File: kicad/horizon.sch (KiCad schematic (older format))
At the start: 105 parts, among them J1 OLED, SW1 SW_Push, SW10 SW_Push, SW11 SW_Push, SW12 SW_Push, SW13 SW_Push, SW14 SW_Push, SW15 SW_Push, SW16 SW_Push, SW17 SW_Push, SW18 SW_Push, SW19 SW_Push, SW2 SW_Push, SW20 SW_Push, SW21 SW_Push, SW22 SW_Push, SW23 SW_Push, SW24 SW_Push, SW25 SW_Push, SW26 SW_Push, SW27 SW_Push, SW28 SW_Push, SW29 SW_Push, SW3 SW_Push, SW30 SW_Push, SW31 SW_Push, SW32 SW_Push, SW33 SW_Push, SW34 SW_Push, SW35 SW_Push, SW36 SW_Push, SW37 SW_Push, SW38 SW_Push, SW39 SW_Push, SW4 SW_Push, SW40 SW_Push, SW41 SW_Push, SW42 SW_Push, SW5 SW_Push, SW6 SW_Push, SW7 SW_Push, SW8 SW_Push, SW9 SW_Push, U1 PRO-MICRO

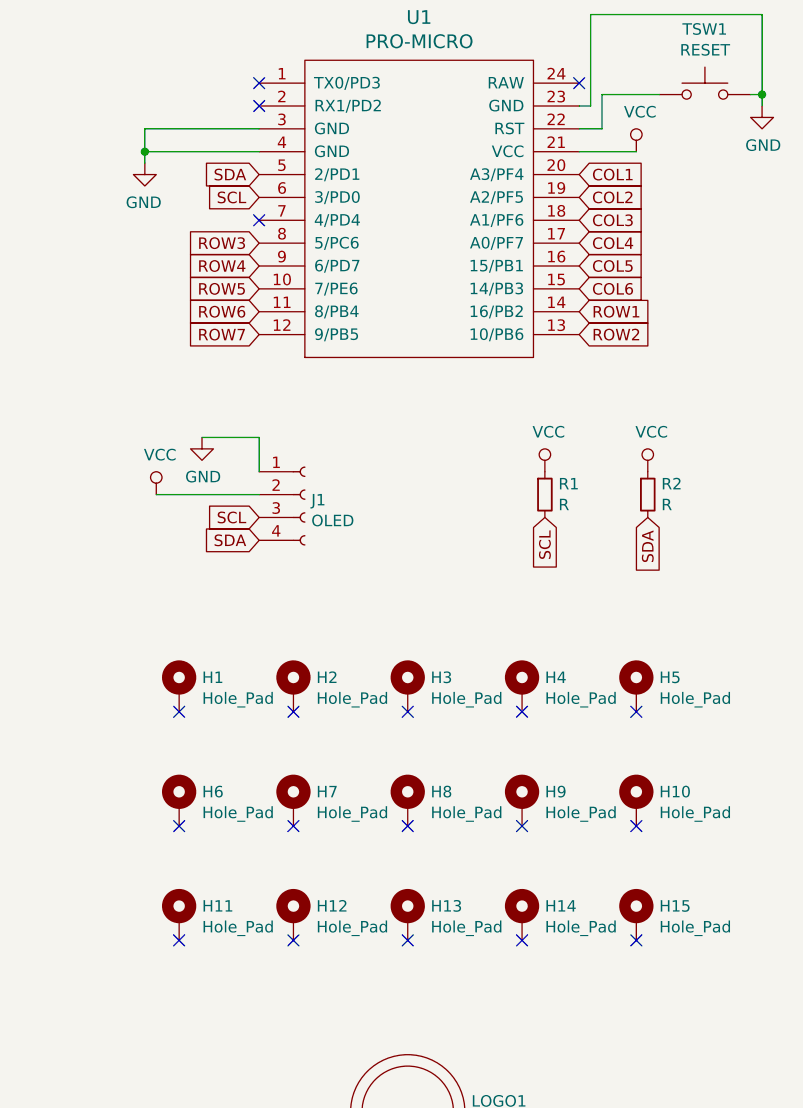
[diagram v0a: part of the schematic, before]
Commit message: Begin revision 2
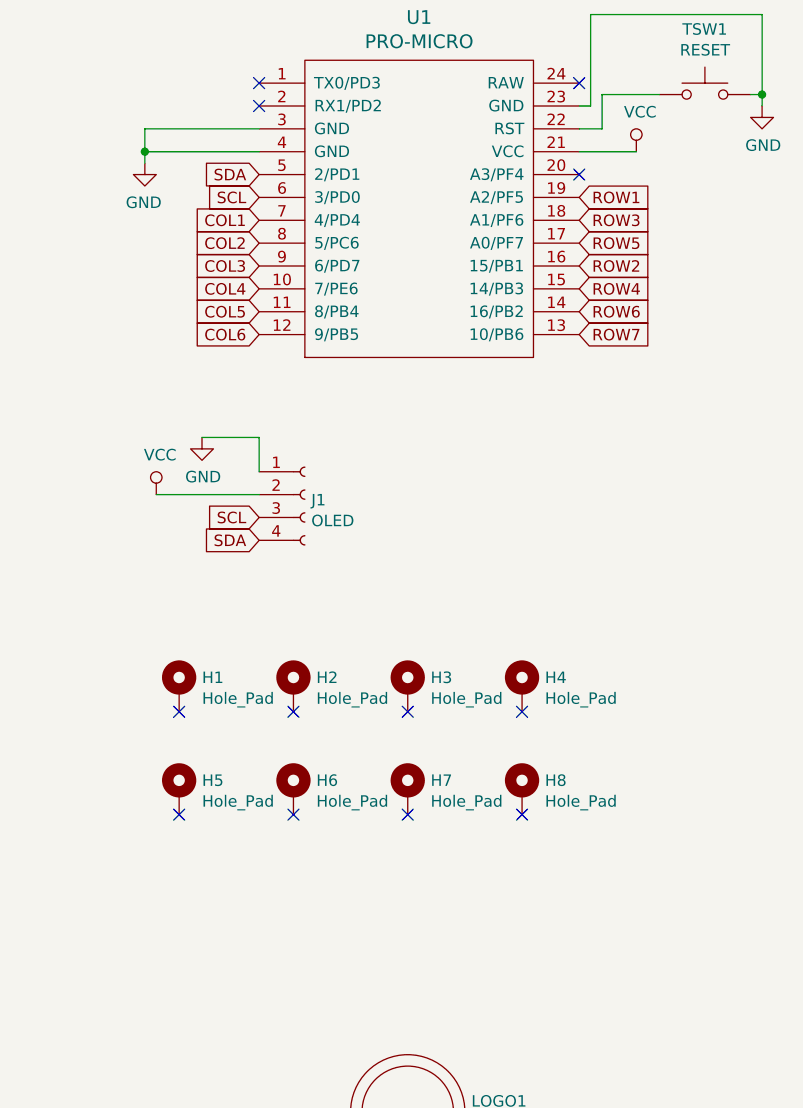
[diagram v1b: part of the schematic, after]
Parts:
- removed H10, H11, H12, H13, H14, H15, H9: Hole_Pad, horizon-footprints:MountingHole_M2, symbol horizon-components:Hole_Pad
- removed R1, R2: R, horizon-footprints:R_0805, symbol horizon-components:R
- D1, D10, D11, D12, D13, D14, D15, D16, D17, D18, D19, D2, D20, D21, D22, D23, D24, D25, D26, D27, D28, D29, D3, D30, D31, D32, D33, D34, D35, D36, D37, D38, D39, D4, D40, D41, D42, D5, D6, D7, D8, D9: footprint horizon-footprints:D_SOD-323 -> horizon-footprints:D_SOD-123
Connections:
- net COL1: now also U1.7 (4/PD4); no longer U1.20 (A3/PF4)
- net COL2: now also U1.8 (5/PC6); no longer U1.19 (A2/PF5)
- net COL3: now also U1.9 (6/PD7); no longer U1.18 (A1/PF6)
- net COL4: now also U1.10 (7/PE6); no longer U1.17 (A0/PF7)
- net COL5: now also U1.11 (8/PB4); no longer U1.16 (15/PB1)
- net COL6: now also U1.12 (9/PB5); no longer U1.15 (14/PB3)
- net ROW1: now also U1.19 (A2/PF5); no longer U1.14 (16/PB2)
- net ROW2: now also U1.16 (15/PB1); no longer U1.13 (10/PB6)
- net ROW3: now also U1.18 (A1/PF6); no longer U1.8 (5/PC6)
- net ROW4: now also U1.15 (14/PB3); no longer U1.9 (6/PD7)
- net ROW5: now also U1.17 (A0/PF7); no longer U1.10 (7/PE6)
- net ROW6: now also U1.14 (16/PB2); no longer U1.11 (8/PB4)
- net ROW7: now also U1.13 (10/PB6); no longer U1.12 (9/PB5)
- no-connect marks 19 -> 12
